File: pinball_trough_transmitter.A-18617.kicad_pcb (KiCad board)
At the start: 2 copper layers, 162.6 x 38.1 mm, 8 parts, among them J1 Conn_01x09_Male

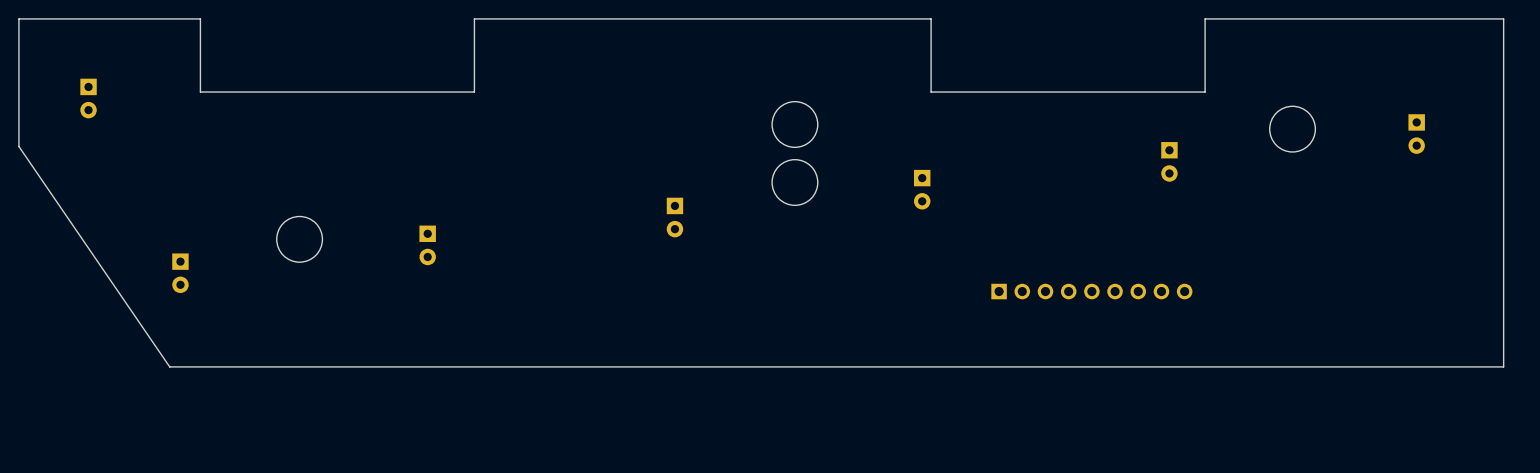
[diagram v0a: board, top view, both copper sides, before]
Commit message: Almost there
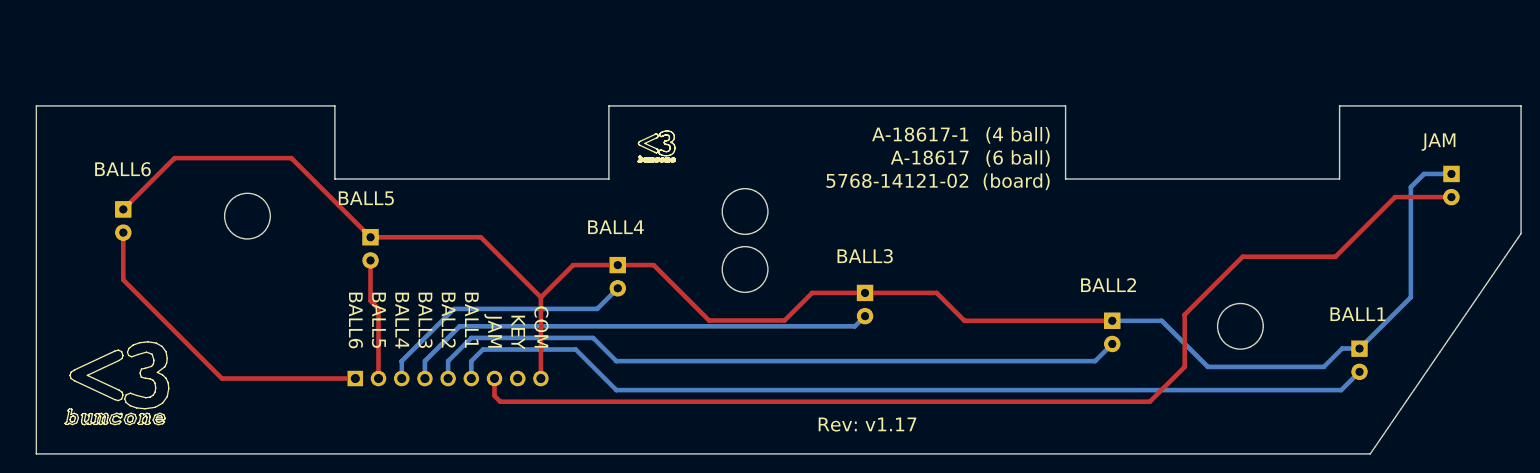
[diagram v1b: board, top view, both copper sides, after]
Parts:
- moved D1 149.5 mm to (218.4, 87.5)
- moved D7 141.9 mm to (73.0, 91.3)
- moved D2 129.4 mm to (208.4, 106.6)
- moved D6 88.0 mm to (100.1, 94.4)
- moved D3 75.6 mm to (181.3, 103.5)
- moved J1 71.1 mm to (98.4, 109.9)
- moved D5 34.7 mm to (127.2, 97.4)
- moved D4 22.9 mm to (154.2, 100.5)
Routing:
- net Net-(D1-Pad1): track 0.00 -> 187.3 mm
- net Net-(D1-Pad2): track 0.00 -> 119.6 mm
- net Net-(D2-Pad2): track 0.00 -> 102.4 mm
- net Net-(D3-Pad2): track 0.00 -> 77.5 mm
- net Net-(D4-Pad2): track 0.00 -> 52.1 mm
- net Net-(D7-Pad2): track 0.00 -> 35.1 mm
- net Net-(D5-Pad2): track 0.00 -> 28.9 mm
- net Net-(D6-Pad2): track 0.00 -> 13.3 mm
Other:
- outline, holes or cut-outs redrawn
- board text added: "(4 ball)"
- board text added: "(6 ball)"
- board text added: "(board)"
- board text added: "5768-14121-02"
- board text added: "A-18617"
- board text added: "A-18617-1"
- board text added: "BALL1"
- board text added: "BALL2"
- board text added: "BALL3"
- board text added: "BALL4"
- board text added: "BALL5"
- board text added: "BALL6"
- board text added: "COM"
- board text added: "COMPONENT SIDE"
- board text added: "JAM"
- board text added: "KEY"
- board text added: "Rev: v1.17"
- board text removed: "Rev: v1.16"
